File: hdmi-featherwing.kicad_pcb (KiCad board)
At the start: 2 copper layers, 22.9 x 50.8 mm, 11 parts, among them J1 HDMI_A

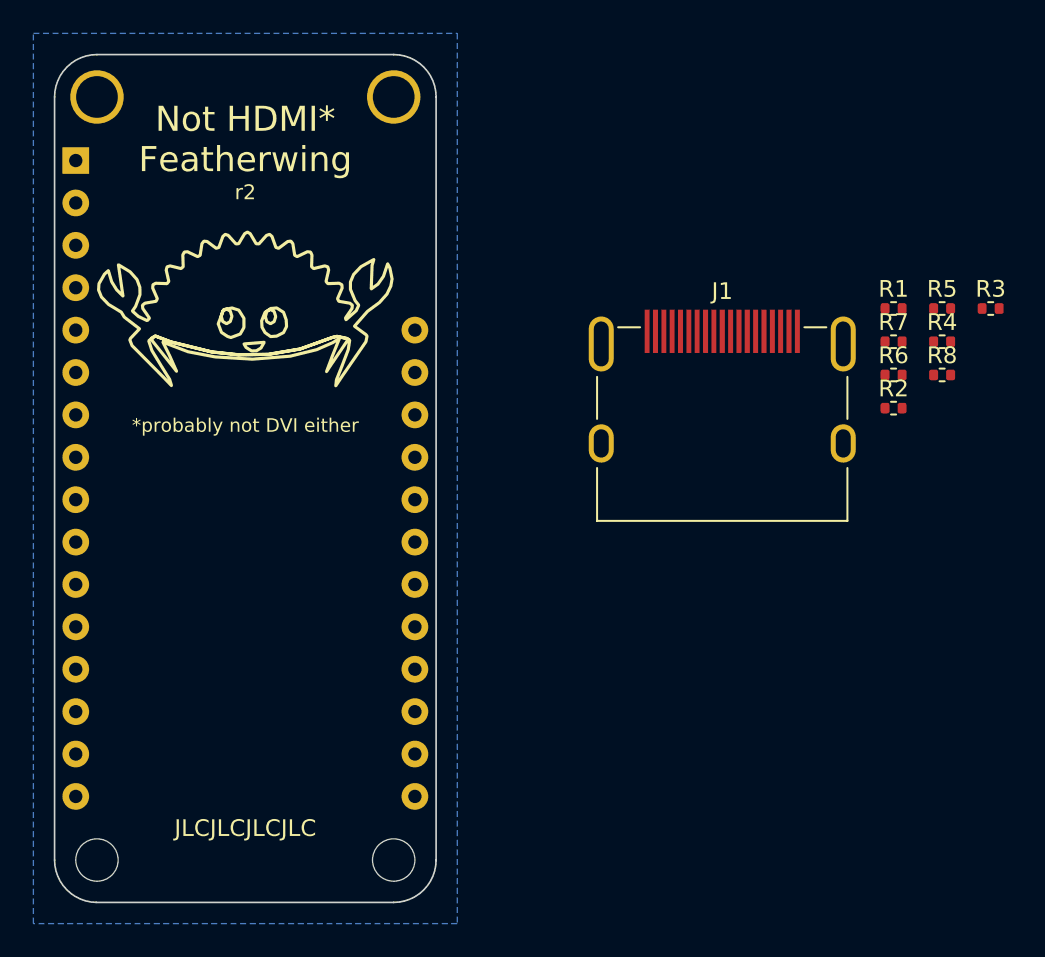
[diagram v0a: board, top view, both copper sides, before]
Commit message: route diffpairs
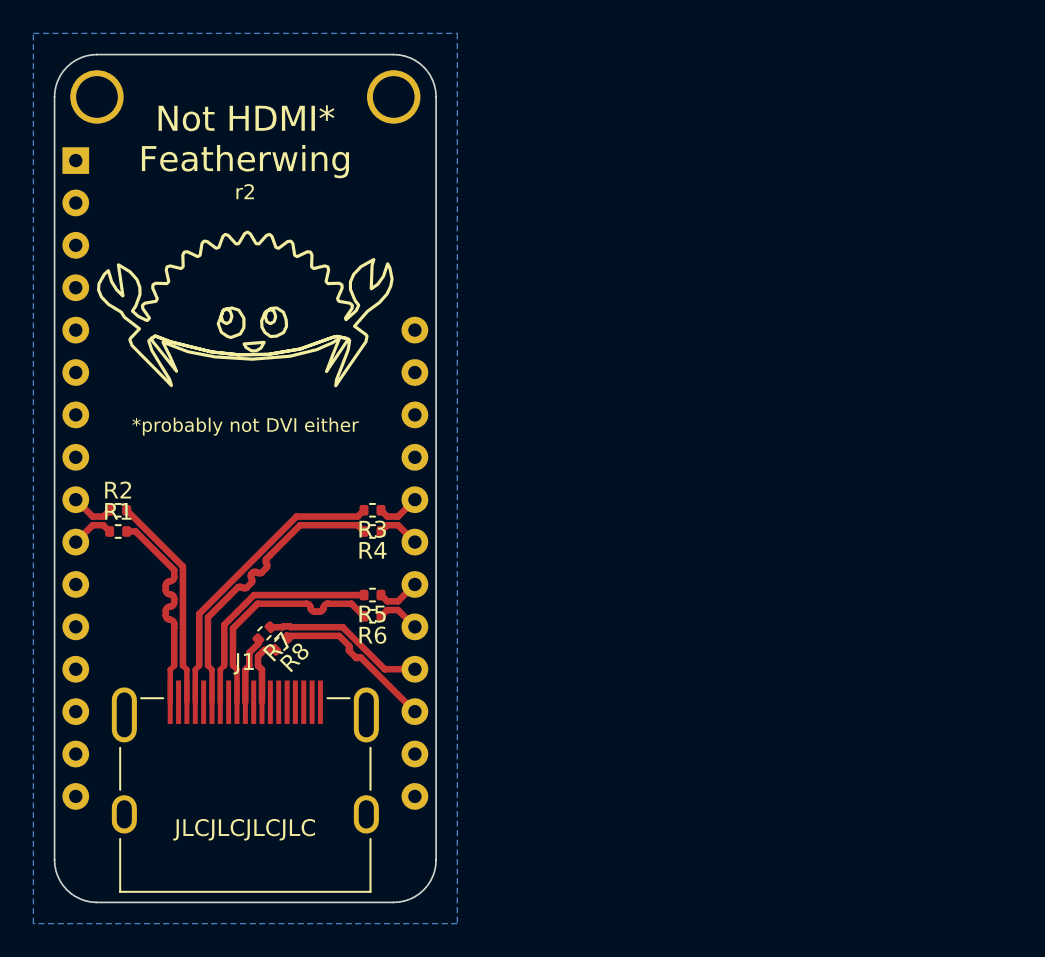
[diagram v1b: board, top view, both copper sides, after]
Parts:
- moved R2 50.8 mm to (111.8, 106.0)
- moved R1 48.3 mm to (111.8, 107.3)
- moved R7 44.2 mm to (120.5, 113.4), turned to -135 degrees
- moved R8 42.7 mm to (121.5, 114.0), turned to -135 degrees
- moved R5 40.8 mm to (127.0, 111.1), turned to 180 degrees
- moved J1 36.2 mm to (119.4, 121.3)
- moved R6 35.3 mm to (127.0, 112.4), turned to 180 degrees
- moved R4 32.6 mm to (127.0, 107.3), turned to 180 degrees
- moved R3 31.8 mm to (127.0, 106.0), turned to 180 degrees
- renumbered R5 to R2, R2 to R3, R6 to R4, R3 to R5, R7 to R6, R4 to R7
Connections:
- A1 pad 10: /WING_CK+ -> /WING_D2+
- A1 pad 19: /WING_D2- -> /WING_CK-
- A1 pad 20: /WING_D2+ -> /WING_CK+
- A1 pad 21: /WING_D1- -> /WING_D0-
- A1 pad 22: /WING_D1+ -> /WING_D0+
- A1 pad 23: /WING_D0- -> /WING_D1-
- A1 pad 24: /WING_D0+ -> /WING_D1+
- A1 pad 9: /WING_CK- -> /WING_D2-
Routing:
- net /D1+: track 0.00 -> 17.8 mm
- net /D1-: track 0.00 -> 17.8 mm
- net /D0+: track 0.00 -> 13.8 mm
- net /D0-: track 0.00 -> 13.8 mm
- net /D2-: track 0.00 -> 13.0 mm
- net /D2+: track 0.00 -> 12.9 mm
- net /WING_CK-: track 0.00 -> 9.79 mm
- net /WING_CK+: track 0.00 -> 9.74 mm
- net /CK+: track 0.00 -> 4.10 mm
- net /CK-: track 0.00 -> 4.05 mm
- net /WING_D2-: track 0.00 -> 2.60 mm
- net /WING_D2+: track 0.00 -> 2.60 mm
- net /WING_D1-: track 0.00 -> 2.60 mm
- net /WING_D1+: track 0.00 -> 2.60 mm
- net /WING_D0-: track 0.00 -> 2.60 mm
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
